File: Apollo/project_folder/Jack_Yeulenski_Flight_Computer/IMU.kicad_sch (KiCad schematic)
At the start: 4 parts, among them U1 BNO055

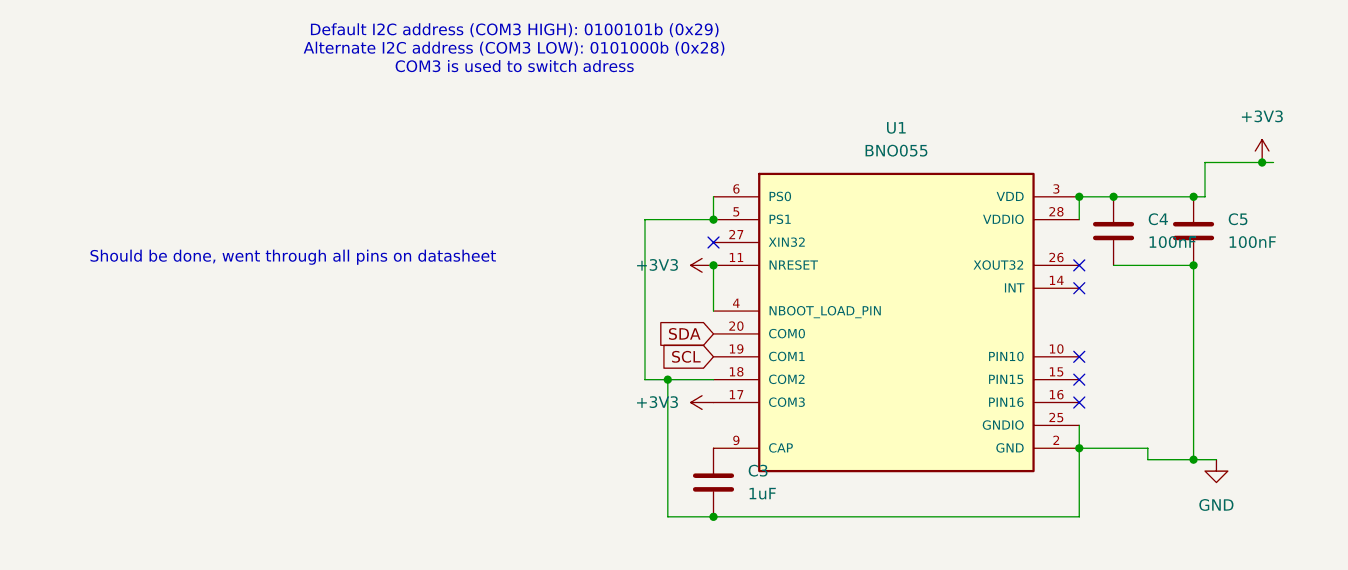
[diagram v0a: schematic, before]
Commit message: Replaced BNO with BMI
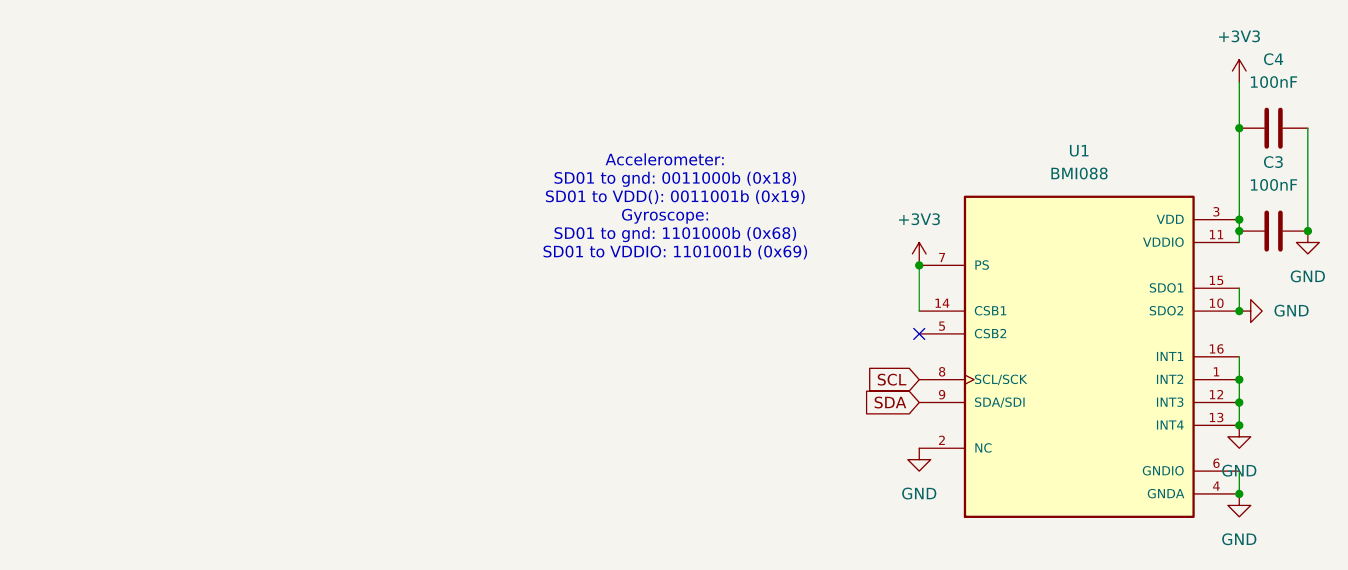
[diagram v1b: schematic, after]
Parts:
- removed C5: 100nF, Capacitor_SMD:C_0805_2012Metric, symbol Device:C
- removed U1: BNO055, Package_LGA:LGA-28_5.2x3.8mm_P0.5mm, symbol SRAD:BNO055
- added U1: BMI088, BMI088 (1):PQFN50P450X300X100-16N, symbol BMI088:BMI088
- C3: value 1uF -> 100nF; footprint Capacitor_SMD:C_0805_2012Metric -> Capacitor_SMD:C_0603_1608Metric
- C4: footprint Capacitor_SMD:C_0805_2012Metric -> Capacitor_SMD:C_0603_1608Metric
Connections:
- net +3V3: now also C3.1, U1.11 (VDDIO), U1.14 (CSB1), U1.3 (VDD), U1.7 (PS)
- net GND: now also C3.2, U1.1 (INT2), U1.10 (SDO2), U1.12 (INT3), U1.13 (INT4), U1.15 (SDO1), U1.16 (INT1), U1.2 (NC), U1.4 (GNDA), U1.6 (GNDIO); no longer C3.1
- net SCL: now also U1.8 (SCL/SCK)
- net SDA: now also U1.9 (SDA/SDI)
- no-connect marks 6 -> 1
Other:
- note added: "Accelerometer: SD01 to gnd: 0011000b (0x18) SD01 to VDD(): 0011001b (0x19) Gyroscope: SD01 to gnd: 1101000b (0x68) SD01 to VDDIO: 1101001b (0x69)"
- note removed: "Default I2C address (COM3 HIGH): 0100101b (0x29) Alternate I2C address (COM3 LOW): 0101000b (0x28) COM3 is used to switch adress"
- note removed: "Should be done, went through all pins on datasheet"
